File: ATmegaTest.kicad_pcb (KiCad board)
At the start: 2 copper layers, 101.6 x 53.3 mm, 18 parts, among them P1 Digital, P10 CONN_01X01, P11 CONN_01X01, P12 CONN_01X01, P13 CONN_01X01, P2 Power, P3 Analog, P4 Analog, P5 PWM, P6 PWM, P7 Communication, P8 CONN_01X01, P9 CONN_01X01, SW1 SW_DIP_x01

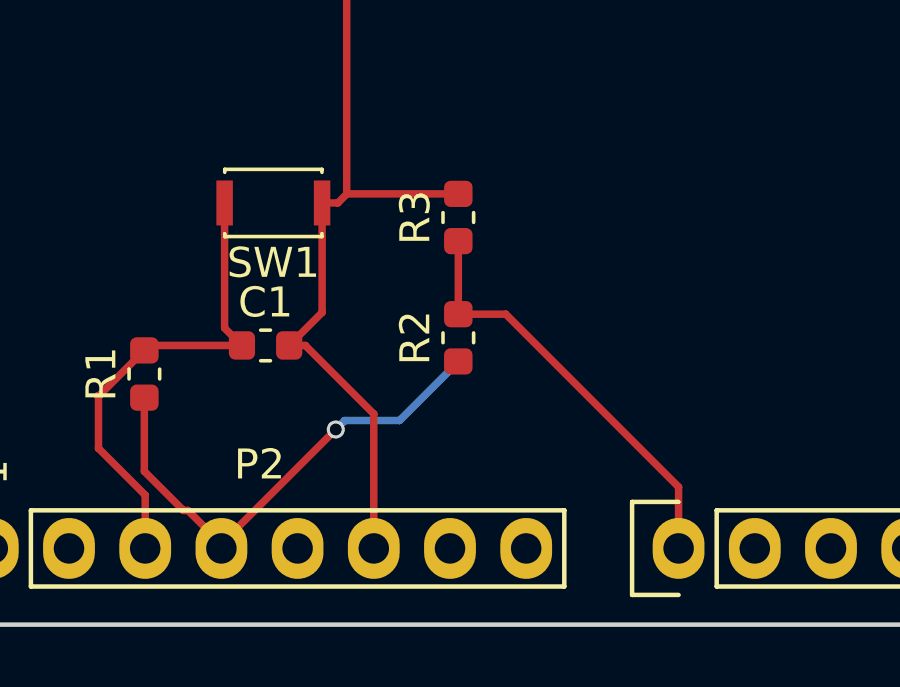
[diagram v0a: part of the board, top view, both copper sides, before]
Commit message: Revert "DividerCkt"
This reverts commit aaad2765e5774504384bd17e4f9678753ffa88e0.
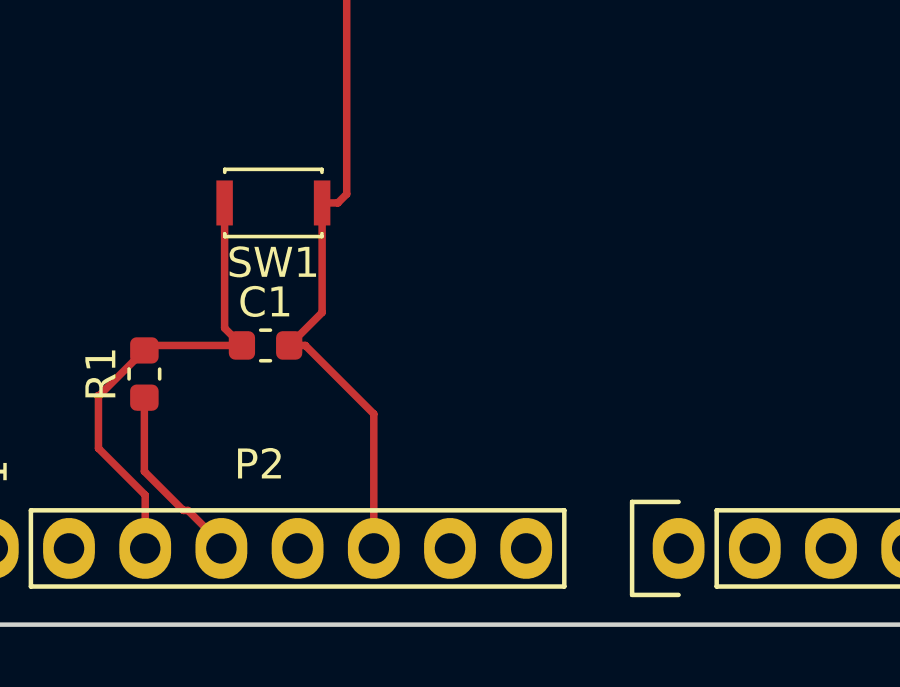
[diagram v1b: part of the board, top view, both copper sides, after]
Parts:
- removed R2, R3: 10k, Resistor_SMD:R_0603_1608Metric
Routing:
- net /A0: track 14.2 -> 0.00 mm
- net +3V3: track 16.6 -> 6.18 mm, vias 1 -> 0
- net GND: track 60.1 -> 56.4 mm
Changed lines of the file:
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@@
     (thickness 1.6)
     (drawings 27)
-    (tracks 38)
+    (tracks 26)
     (zones 0)
-    (modules 18)
+    (modules 16)
     (nets 87)
   )
@@
     (add_net "Net-(P9-Pad1)")
   )
-  (module Resistor_SMD:R_0603_1608Metric (layer F.Cu)
-    (at 146.835001 108.094999 90)
-    (descr "Resistor SMD 0603 (1608 Metric), square (rectangular) end terminal, IPC_7351 nominal, (Body size source: http://www.tortai-tech.com/upload/download/2011102023233369053.pdf), generated with kicad-footprint-generator")
-    (tags resistor)
-    (attr smd)
-    (fp_text reference R3 (at 0 -1.43 90) (layer F.SilkS)
-      (effects (font (size 1 1) (thickness 0.15)))
-    )
-    (fp_text value 10k (at 0 1.43 90) (layer F.Fab)
-      (effects (font (size 1 1) (thickness 0.15)))
-    )
-    (fp_text user %R (at 0 0 90) (layer F.Fab)
-      (effects (font (size 0.4 0.4) (thickness 0.06)))
-    )
-    (fp_line (start 1.48 0.73) (end -1.48 0.73) (layer F.CrtYd) (width 0.05))
-    (fp_line (start 1.48 -0.73) (end 1.48 0.73) (layer F.CrtYd) (width 0.05))
-    (fp_line (start -1.48 -0.73) (end 1.48 -0.73) (layer F.CrtYd) (width 0.05))
-    (fp_line (start -1.48 0.73) (end -1.48 -0.73) (layer F.CrtYd) (width 0.05))
-    (fp_line (start -0.162779 0.51) (end 0.162779 0.51) (layer F.SilkS) (width 0.12))
-    (fp_line (start -0.162779 -0.51) (end 0.162779 -0.51) (layer F.SilkS) (width 0.12))
-    (fp_line (start 0.8 0.4) (end -0.8 0.4) (layer F.Fab) (width 0.1))
-    (fp_line (start 0.8 -0.4) (end 0.8 0.4) (layer F.Fab) (width 0.1))
-    (fp_line (start -0.8 -0.4) (end 0.8 -0.4) (layer F.Fab) (width 0.1))
-    (fp_line (start -0.8 0.4) (end -0.8 -0.4) (layer F.Fab) (width 0.1))
-    (pad 2 smd roundrect (at 0.7875 0 90) (size 0.875 0.95) (layers F.Cu F.Paste F.Mask) (roundrect_rratio 0.25)
-      (net 1 GND))
-    (pad 1 smd roundrect (at -0.7875 0 90) (size 0.875 0.95) (layers F.Cu F.Paste F.Mask) (roundrect_rratio 0.25)
-      (net 38 /A0))
-    (model ${KISYS3DMOD}/Resistor_SMD.3dshapes/R_0603_1608Metric.wrl
-      (at (xyz 0 0 0))
-      (scale (xyz 1 1 1))
-      (rotate (xyz 0 0 0))
-    )
-  )
-  (module Resistor_SMD:R_0603_1608Metric (layer F.Cu)
-    (at 146.835001 112.104999 90)
-    (descr "Resistor SMD 0603 (1608 Metric), square (rectangular) end terminal, IPC_7351 nominal, (Body size source: http://www.tortai-tech.com/upload/download/2011102023233369053.pdf), generated with kicad-footprint-generator")
-    (tags resistor)
-    (attr smd)
-    (fp_text reference R2 (at 0 -1.43 90) (layer F.SilkS)
-      (effects (font (size 1 1) (thickness 0.15)))
-    )
-    (fp_text value 10k (at 0 1.43 90) (layer F.Fab)
-      (effects (font (size 1 1) (thickness 0.15)))
-    )
-    (fp_text user %R (at 0 0 90) (layer F.Fab)
-      (effects (font (size 0.4 0.4) (thickness 0.06)))
-    )
-    (fp_line (start 1.48 0.73) (end -1.48 0.73) (layer F.CrtYd) (width 0.05))
-    (fp_line (start 1.48 -0.73) (end 1.48 0.73) (layer F.CrtYd) (width 0.05))
-    (fp_line (start -1.48 -0.73) (end 1.48 -0.73) (layer F.CrtYd) (width 0.05))
-    (fp_line (start -1.48 0.73) (end -1.48 -0.73) (layer F.CrtYd) (width 0.05))
-    (fp_line (start -0.162779 0.51) (end 0.162779 0.51) (layer F.SilkS) (width 0.12))
-    (fp_line (start -0.162779 -0.51) (end 0.162779 -0.51) (layer F.SilkS) (width 0.12))
-    (fp_line (start 0.8 0.4) (end -0.8 0.4) (layer F.Fab) (width 0.1))
-    (fp_line (start 0.8 -0.4) (end 0.8 0.4) (layer F.Fab) (width 0.1))
-    (fp_line (start -0.8 -0.4) (end 0.8 -0.4) (layer F.Fab) (width 0.1))
-    (fp_line (start -0.8 0.4) (end -0.8 -0.4) (layer F.Fab) (width 0.1))
-    (pad 2 smd roundrect (at 0.7875 0 90) (size 0.875 0.95) (layers F.Cu F.Paste F.Mask) (roundrect_rratio 0.25)
-      (net 38 /A0))
-    (pad 1 smd roundrect (at -0.7875 0 90) (size 0.875 0.95) (layers F.Cu F.Paste F.Mask) (roundrect_rratio 0.25)
-      (net 78 +3V3))
-    (model ${KISYS3DMOD}/Resistor_SMD.3dshapes/R_0603_1608Metric.wrl
-      (at (xyz 0 0 0))
-      (scale (xyz 1 1 1))
-      (rotate (xyz 0 0 0))
-    )
-  )
   (module Button_Switch_SMD:SW_SPST_CK_KXT3 (layer F.Cu)
     (at 140.67 107.61 180)
@@
   (segment (start 142.82 107.61) (end 143.115001 107.314999) (width 0.25) (layer F.Cu) (net 1))
   (segment (start 142.295 107.61) (end 142.82 107.61) (width 0.25) (layer F.Cu) (net 1))
-  (segment (start 143.122501 107.307499) (end 146.835001 107.307499) (width 0.25) (layer F.Cu) (net 1))
-  (segment (start 143.115001 107.314999) (end 143.122501 107.307499) (width 0.25) (layer F.Cu) (net 1))
   (segment (start 139.045 111.7825) (end 139.6225 112.36) (width 0.25) (layer F.Cu) (net 36))
   (segment (start 139.045 107.61) (end 139.045 111.7825) (width 0.25) (layer F.Cu) (net 36))
@@
   (segment (start 136.398 119.126) (end 136.398 117.348) (width 0.25) (layer F.Cu) (net 36))
   (segment (start 136.398 117.348) (end 134.84 115.79) (width 0.25) (layer F.Cu) (net 36))
-  (segment (start 146.835001 108.882499) (end 146.835001 111.317499) (width 0.25) (layer F.Cu) (net 38))
-  (segment (start 146.835001 111.317499) (end 148.417499 111.317499) (width 0.25) (layer F.Cu) (net 38))
-  (segment (start 154.178 117.078) (end 154.178 119.126) (width 0.25) (layer F.Cu) (net 38))
-  (segment (start 148.417499 111.317499) (end 154.178 117.078) (width 0.25) (layer F.Cu) (net 38))
   (segment (start 138.938 118.9736) (end 138.938 119.126) (width 0.25) (layer F.Cu) (net 78))
   (segment (start 137.8244 117.86) (end 138.938 118.9736) (width 0.25) (layer F.Cu) (net 78))
@@
   (segment (start 136.37 116.558) (end 137.672 117.86) (width 0.25) (layer F.Cu) (net 78))
   (segment (start 136.37 114.1) (end 136.37 116.558) (width 0.25) (layer F.Cu) (net 78))
-  (segment (start 138.938 118.9736) (end 142.75 115.1616) (width 0.25) (layer F.Cu) (net 78))
-  (segment (start 142.75 115.1616) (end 142.75 115.1616) (width 0.25) (layer F.Cu) (net 78))
-  (via (at 142.75 115.1616) (size 0.6) (drill 0.4) (layers F.Cu B.Cu) (net 78))
-  (segment (start 143.049999 114.861601) (end 144.878399 114.861601) (width 0.25) (layer B.Cu) (net 78))
-  (segment (start 142.75 115.1616) (end 143.049999 114.861601) (width 0.25) (layer B.Cu) (net 78))
-  (segment (start 144.878399 114.861601) (end 146.83 112.91) (width 0.25) (layer B.Cu) (net 78))
 )

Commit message: DividerCkt
PCB changes as per SchematicDividerCkt
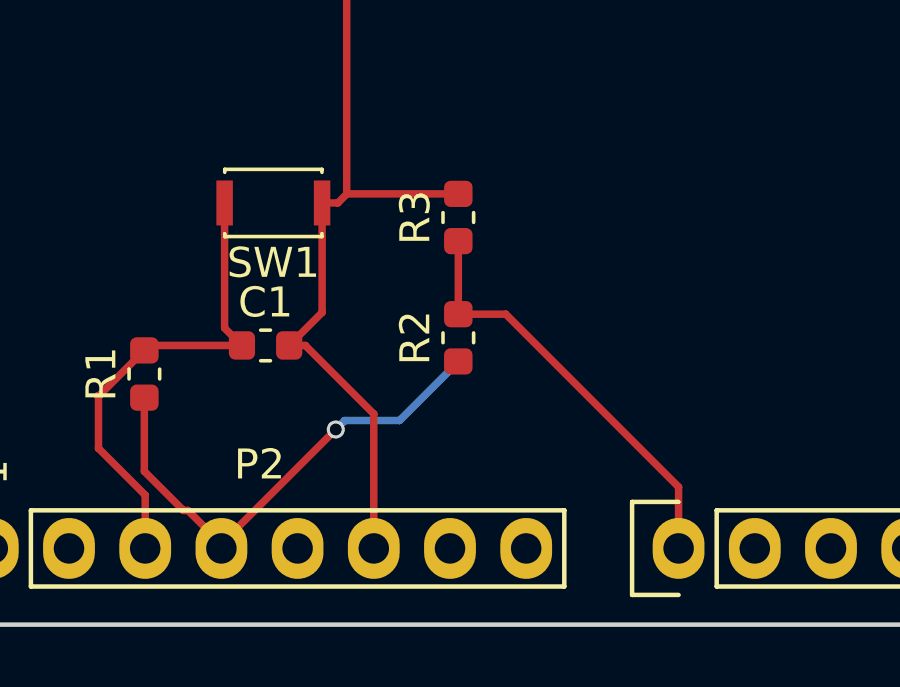
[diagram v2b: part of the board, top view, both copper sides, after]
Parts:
- added R2: 10k, Resistor_SMD:R_0603_1608Metric, F.Cu at (146.8, 112.1)
- added R3: 10k, Resistor_SMD:R_0603_1608Metric, F.Cu at (146.8, 108.1)
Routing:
- net /A0: track 0.00 -> 14.2 mm
- net +3V3: track 6.18 -> 16.6 mm, vias 0 -> 1
- net GND: track 56.4 -> 60.1 mm
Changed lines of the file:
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@@
     (thickness 1.6)
     (drawings 27)
-    (tracks 26)
+    (tracks 38)
     (zones 0)
-    (modules 16)
+    (modules 18)
     (nets 87)
   )
@@
     (add_net "Net-(P9-Pad1)")
   )
+  (module Resistor_SMD:R_0603_1608Metric (layer F.Cu)
+    (at 146.835001 108.094999 90)
+    (descr "Resistor SMD 0603 (1608 Metric), square (rectangular) end terminal, IPC_7351 nominal, (Body size source: http://www.tortai-tech.com/upload/download/2011102023233369053.pdf), generated with kicad-footprint-generator")
+    (tags resistor)
+    (attr smd)
+    (fp_text reference R3 (at 0 -1.43 90) (layer F.SilkS)
+      (effects (font (size 1 1) (thickness 0.15)))
+    )
+    (fp_text value 10k (at 0 1.43 90) (layer F.Fab)
+      (effects (font (size 1 1) (thickness 0.15)))
+    )
+    (fp_text user %R (at 0 0 90) (layer F.Fab)
+      (effects (font (size 0.4 0.4) (thickness 0.06)))
+    )
+    (fp_line (start 1.48 0.73) (end -1.48 0.73) (layer F.CrtYd) (width 0.05))
+    (fp_line (start 1.48 -0.73) (end 1.48 0.73) (layer F.CrtYd) (width 0.05))
+    (fp_line (start -1.48 -0.73) (end 1.48 -0.73) (layer F.CrtYd) (width 0.05))
+    (fp_line (start -1.48 0.73) (end -1.48 -0.73) (layer F.CrtYd) (width 0.05))
+    (fp_line (start -0.162779 0.51) (end 0.162779 0.51) (layer F.SilkS) (width 0.12))
+    (fp_line (start -0.162779 -0.51) (end 0.162779 -0.51) (layer F.SilkS) (width 0.12))
+    (fp_line (start 0.8 0.4) (end -0.8 0.4) (layer F.Fab) (width 0.1))
+    (fp_line (start 0.8 -0.4) (end 0.8 0.4) (layer F.Fab) (width 0.1))
+    (fp_line (start -0.8 -0.4) (end 0.8 -0.4) (layer F.Fab) (width 0.1))
+    (fp_line (start -0.8 0.4) (end -0.8 -0.4) (layer F.Fab) (width 0.1))
+    (pad 2 smd roundrect (at 0.7875 0 90) (size 0.875 0.95) (layers F.Cu F.Paste F.Mask) (roundrect_rratio 0.25)
+      (net 1 GND))
+    (pad 1 smd roundrect (at -0.7875 0 90) (size 0.875 0.95) (layers F.Cu F.Paste F.Mask) (roundrect_rratio 0.25)
+      (net 38 /A0))
+    (model ${KISYS3DMOD}/Resistor_SMD.3dshapes/R_0603_1608Metric.wrl
+      (at (xyz 0 0 0))
+      (scale (xyz 1 1 1))
+      (rotate (xyz 0 0 0))
+    )
+  )
+  (module Resistor_SMD:R_0603_1608Metric (layer F.Cu)
+    (at 146.835001 112.104999 90)
+    (descr "Resistor SMD 0603 (1608 Metric), square (rectangular) end terminal, IPC_7351 nominal, (Body size source: http://www.tortai-tech.com/upload/download/2011102023233369053.pdf), generated with kicad-footprint-generator")
+    (tags resistor)
+    (attr smd)
+    (fp_text reference R2 (at 0 -1.43 90) (layer F.SilkS)
+      (effects (font (size 1 1) (thickness 0.15)))
+    )
+    (fp_text value 10k (at 0 1.43 90) (layer F.Fab)
+      (effects (font (size 1 1) (thickness 0.15)))
+    )
+    (fp_text user %R (at 0 0 90) (layer F.Fab)
+      (effects (font (size 0.4 0.4) (thickness 0.06)))
+    )
+    (fp_line (start 1.48 0.73) (end -1.48 0.73) (layer F.CrtYd) (width 0.05))
+    (fp_line (start 1.48 -0.73) (end 1.48 0.73) (layer F.CrtYd) (width 0.05))
+    (fp_line (start -1.48 -0.73) (end 1.48 -0.73) (layer F.CrtYd) (width 0.05))
+    (fp_line (start -1.48 0.73) (end -1.48 -0.73) (layer F.CrtYd) (width 0.05))
+    (fp_line (start -0.162779 0.51) (end 0.162779 0.51) (layer F.SilkS) (width 0.12))
+    (fp_line (start -0.162779 -0.51) (end 0.162779 -0.51) (layer F.SilkS) (width 0.12))
+    (fp_line (start 0.8 0.4) (end -0.8 0.4) (layer F.Fab) (width 0.1))
+    (fp_line (start 0.8 -0.4) (end 0.8 0.4) (layer F.Fab) (width 0.1))
+    (fp_line (start -0.8 -0.4) (end 0.8 -0.4) (layer F.Fab) (width 0.1))
+    (fp_line (start -0.8 0.4) (end -0.8 -0.4) (layer F.Fab) (width 0.1))
+    (pad 2 smd roundrect (at 0.7875 0 90) (size 0.875 0.95) (layers F.Cu F.Paste F.Mask) (roundrect_rratio 0.25)
+      (net 38 /A0))
+    (pad 1 smd roundrect (at -0.7875 0 90) (size 0.875 0.95) (layers F.Cu F.Paste F.Mask) (roundrect_rratio 0.25)
+      (net 78 +3V3))
+    (model ${KISYS3DMOD}/Resistor_SMD.3dshapes/R_0603_1608Metric.wrl
+      (at (xyz 0 0 0))
+      (scale (xyz 1 1 1))
+      (rotate (xyz 0 0 0))
+    )
+  )
   (module Button_Switch_SMD:SW_SPST_CK_KXT3 (layer F.Cu)
     (at 140.67 107.61 180)
@@
   (segment (start 142.82 107.61) (end 143.115001 107.314999) (width 0.25) (layer F.Cu) (net 1))
   (segment (start 142.295 107.61) (end 142.82 107.61) (width 0.25) (layer F.Cu) (net 1))
+  (segment (start 143.122501 107.307499) (end 146.835001 107.307499) (width 0.25) (layer F.Cu) (net 1))
+  (segment (start 143.115001 107.314999) (end 143.122501 107.307499) (width 0.25) (layer F.Cu) (net 1))
   (segment (start 139.045 111.7825) (end 139.6225 112.36) (width 0.25) (layer F.Cu) (net 36))
   (segment (start 139.045 107.61) (end 139.045 111.7825) (width 0.25) (layer F.Cu) (net 36))
@@
   (segment (start 136.398 119.126) (end 136.398 117.348) (width 0.25) (layer F.Cu) (net 36))
   (segment (start 136.398 117.348) (end 134.84 115.79) (width 0.25) (layer F.Cu) (net 36))
+  (segment (start 146.835001 108.882499) (end 146.835001 111.317499) (width 0.25) (layer F.Cu) (net 38))
+  (segment (start 146.835001 111.317499) (end 148.417499 111.317499) (width 0.25) (layer F.Cu) (net 38))
+  (segment (start 154.178 117.078) (end 154.178 119.126) (width 0.25) (layer F.Cu) (net 38))
+  (segment (start 148.417499 111.317499) (end 154.178 117.078) (width 0.25) (layer F.Cu) (net 38))
   (segment (start 138.938 118.9736) (end 138.938 119.126) (width 0.25) (layer F.Cu) (net 78))
   (segment (start 137.8244 117.86) (end 138.938 118.9736) (width 0.25) (layer F.Cu) (net 78))
@@
   (segment (start 136.37 116.558) (end 137.672 117.86) (width 0.25) (layer F.Cu) (net 78))
   (segment (start 136.37 114.1) (end 136.37 116.558) (width 0.25) (layer F.Cu) (net 78))
+  (segment (start 138.938 118.9736) (end 142.75 115.1616) (width 0.25) (layer F.Cu) (net 78))
+  (segment (start 142.75 115.1616) (end 142.75 115.1616) (width 0.25) (layer F.Cu) (net 78))
+  (via (at 142.75 115.1616) (size 0.6) (drill 0.4) (layers F.Cu B.Cu) (net 78))
+  (segment (start 143.049999 114.861601) (end 144.878399 114.861601) (width 0.25) (layer B.Cu) (net 78))
+  (segment (start 142.75 115.1616) (end 143.049999 114.861601) (width 0.25) (layer B.Cu) (net 78))
+  (segment (start 144.878399 114.861601) (end 146.83 112.91) (width 0.25) (layer B.Cu) (net 78))
 )
